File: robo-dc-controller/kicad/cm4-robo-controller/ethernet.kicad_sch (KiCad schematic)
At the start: 6 parts, among them U7 TPD4EUSB30DQAR, U8 TPD4EUSB30DQAR

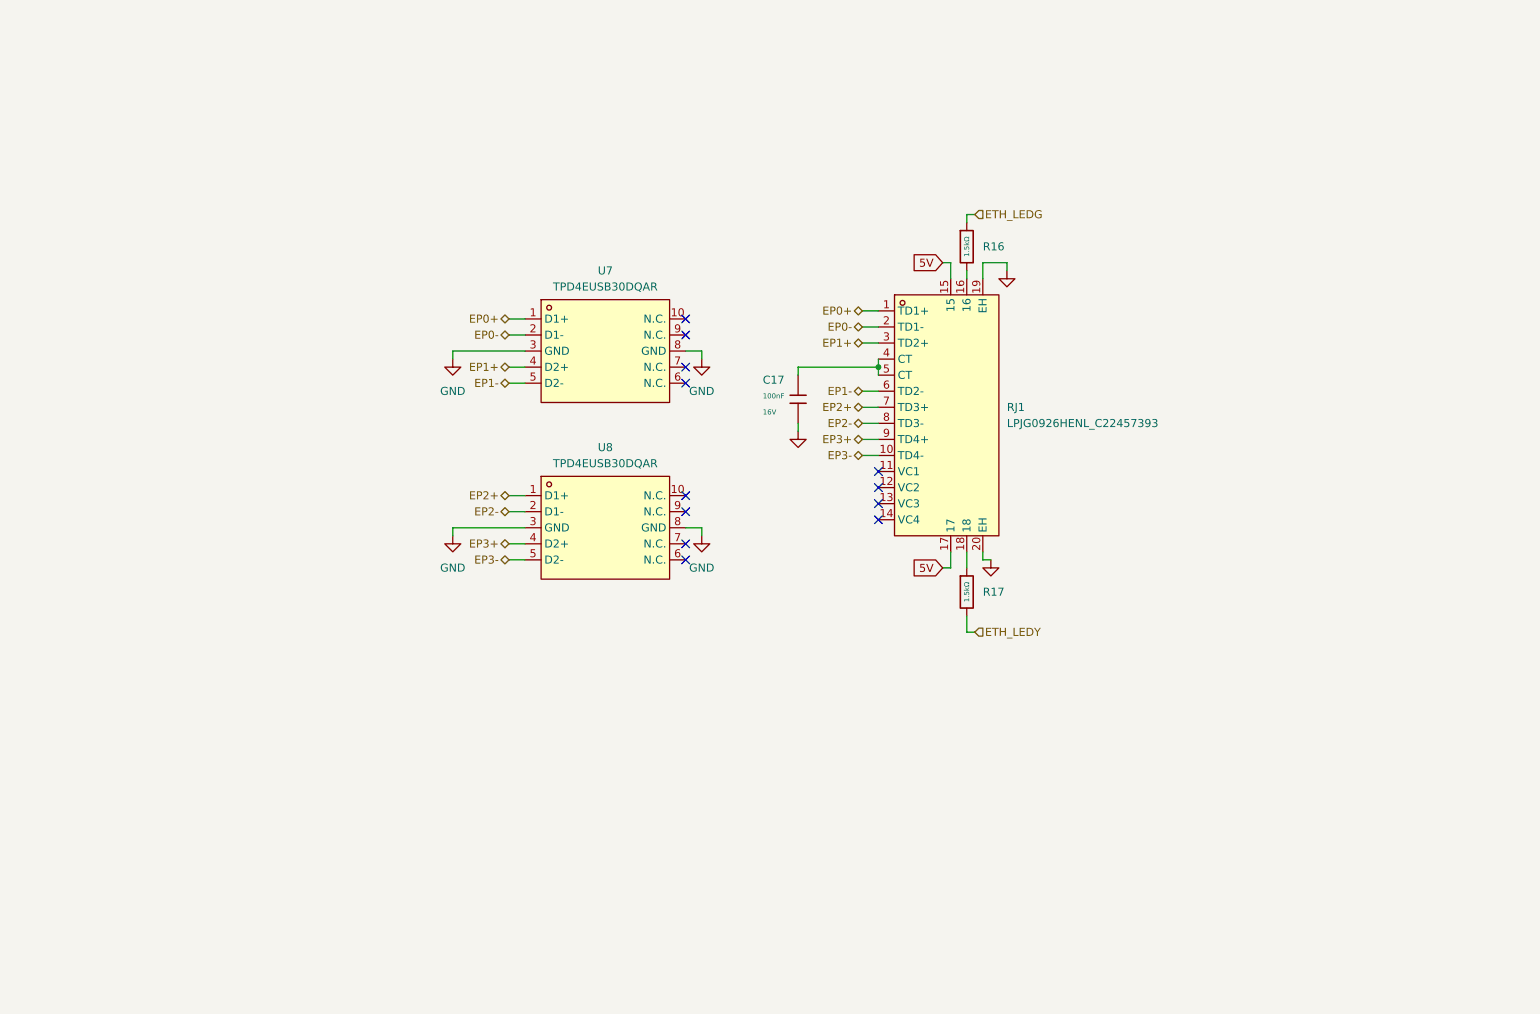
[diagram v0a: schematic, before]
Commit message: Latest ethernet changes
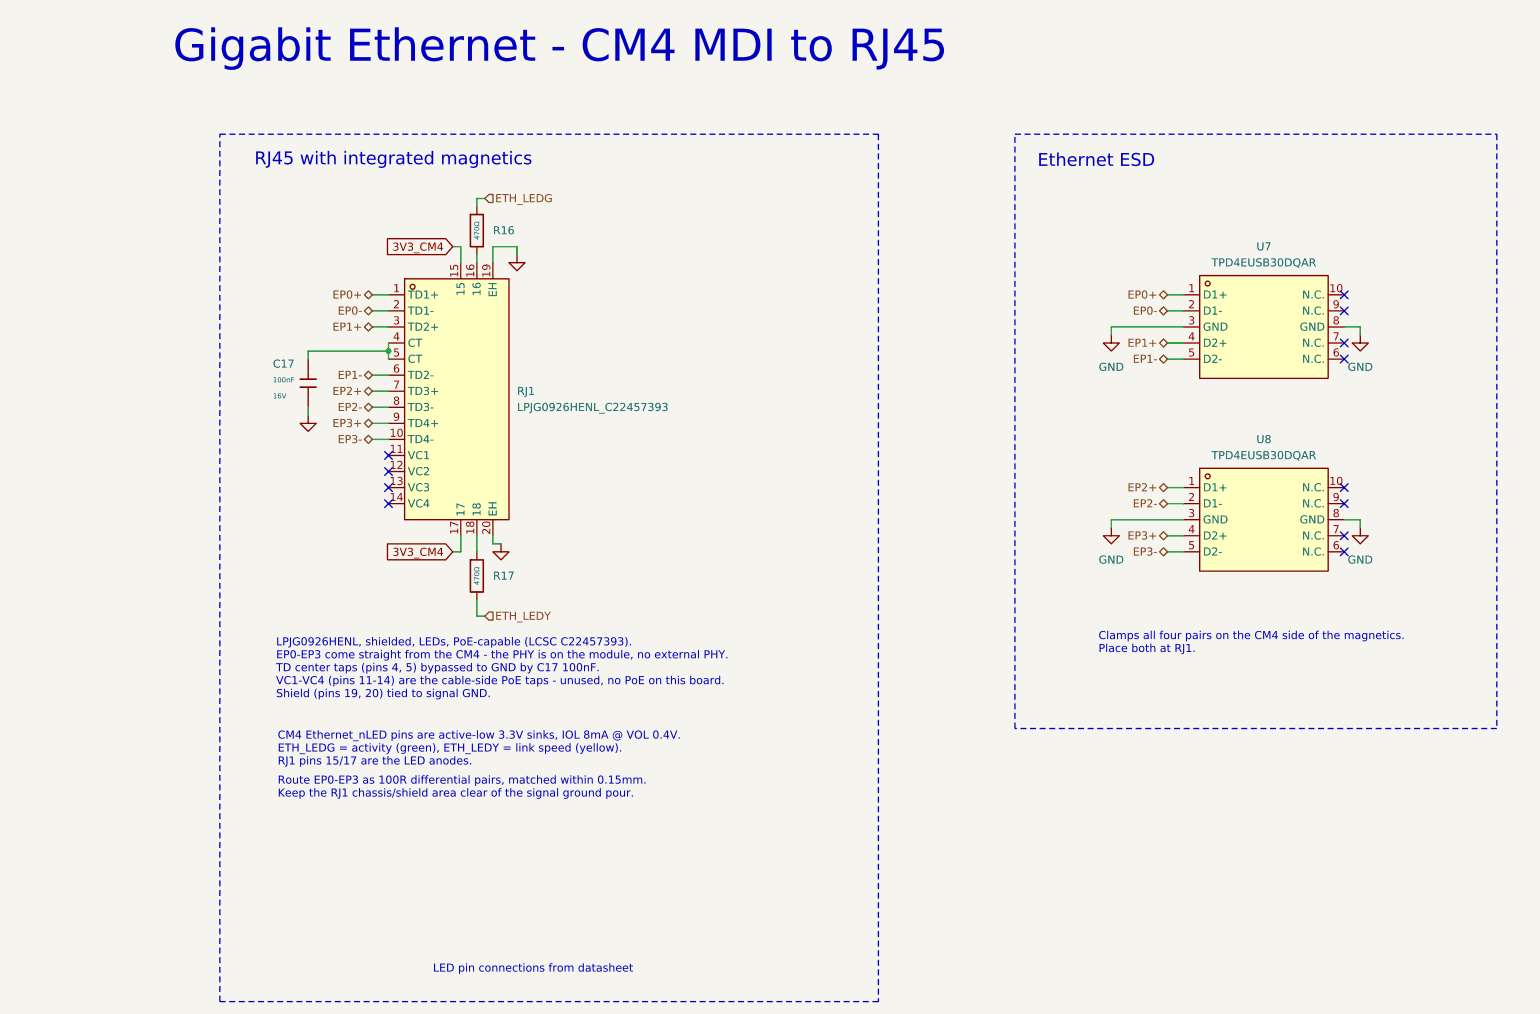
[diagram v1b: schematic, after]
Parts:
- removed R16, R17: 1.5kΩ, PCM_JLCPCB:R_0402, symbol PCM_JLCPCB-Resistors:0402,1.5kΩ
- added R16, R17: 470Ω, PCM_JLCPCB:R_0402, symbol PCM_JLCPCB-Resistors:0402,470Ω
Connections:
- net ETH_LEDG: now also R16.1
- net ETH_LEDY: now also R17.2
- net at RJ1.16: now also R16.2
- net at RJ1.18: now also R17.1
- net 5V renamed 3V3_CM4
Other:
- note added: "CM4 Ethernet_nLED pins are active-low 3.3V sinks, IOL 8mA @ VOL 0.4V. ETH_LEDG = activity (green), ETH_LEDY = link speed (yellow). RJ1 pins 15/17 are the LED anodes."
- note added: "Clamps all four pairs on the CM4 side of the magnetics. Place both at RJ1."
- note added: "Ethernet ESD"
- note added: "Gigabit Ethernet - CM4 MDI to RJ45"
- note added: "LED pin connections from datasheet"
- note added: "LPJG0926HENL, shielded, LEDs, PoE-capable (LCSC C22457393). EP0-EP3 come straight from the CM4 - the PHY is on the module, no external PHY. TD center taps (pins 4, 5) bypassed to GND by C17 100nF. VC1-VC4 (pins 11-14) are the cable-side PoE taps - unused, no PoE on this board. Shield (pins 19, 20) tied to signal GND."
- note added: "RJ45 with integrated magnetics"
- note added: "Route EP0-EP3 as 100R differential pairs, matched within 0.15mm. Keep the RJ1 chassis/shield area clear of the signal ground pour."
- moved on the sheet: C17, RJ1, U7, U8
